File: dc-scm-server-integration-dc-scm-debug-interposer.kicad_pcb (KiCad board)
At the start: 6 copper layers, 90 x 62.3 mm, 166 parts, among them J1 Socket_DC-SCM-2.1_2x84_Rev-1-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, J10 PinHeader_2x5_P2.54mm_SMD, J11 PinHeader_2x5_P2.54mm_SMD, J12 PinHeader_2x5_P2.54mm_SMD, J13 PinHeader_2x5_P2.54mm_SMD, J15 Socket_SOP2-16_ACA-SPI-006-K0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, J16 Socket_SOP2-16_ACA-SPI-006-K0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, J17 PinHeader_2x5_P2.54mm_SMD, J2 PCB-Edge_DC-SCM-2.1_2x84_Rev-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, J3 PinHeader_2x5_P2.54mm_SMD, J4 PinHeader_2x5_P2.54mm_SMD, J5 PinHeader_2x5_P2.54mm_SMD, J6 PinHeader_2x5_P2.54mm_SMD, J7 PinHeader_2x5_P2.54mm_SMD, J9 PinHeader_2x5_P2.54mm_SMD, Q3 DMG1012T-7, U1 TLV76701_WSON

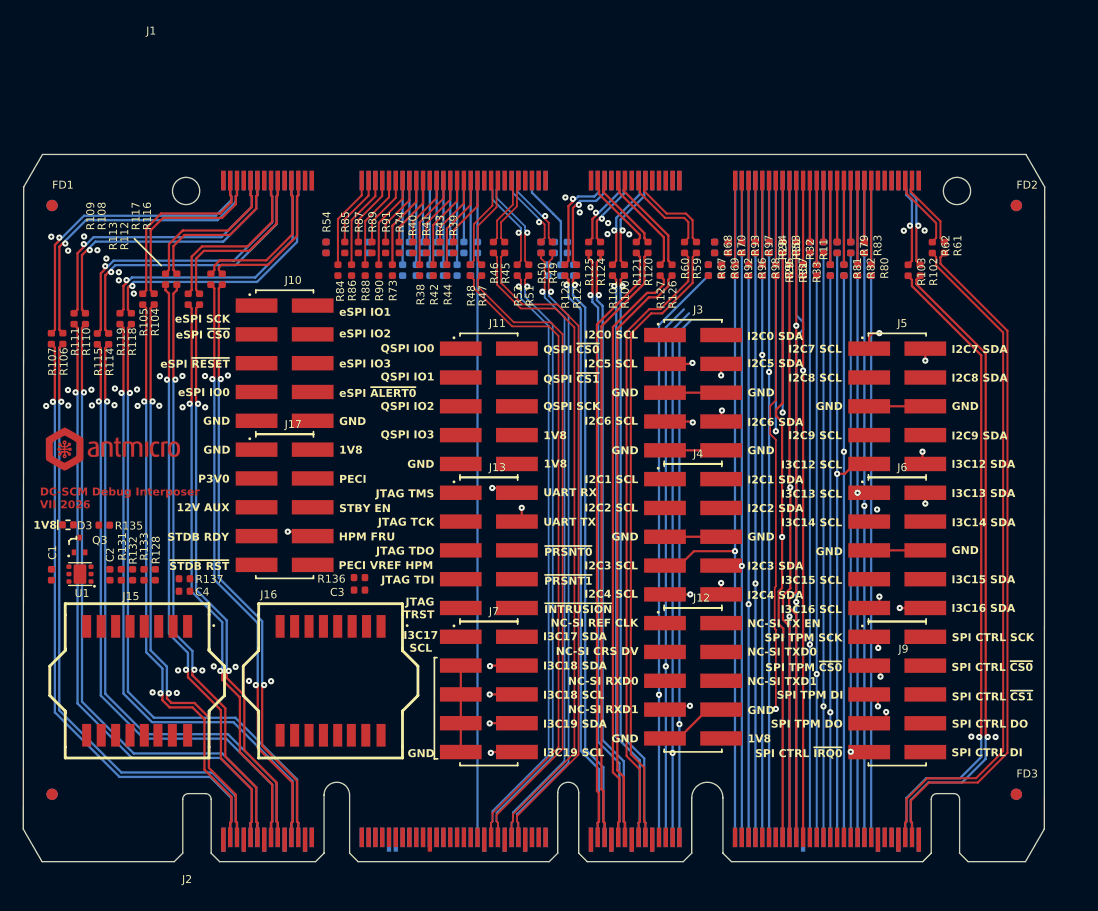
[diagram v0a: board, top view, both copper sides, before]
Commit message: [#100720] Continue routing low speeds
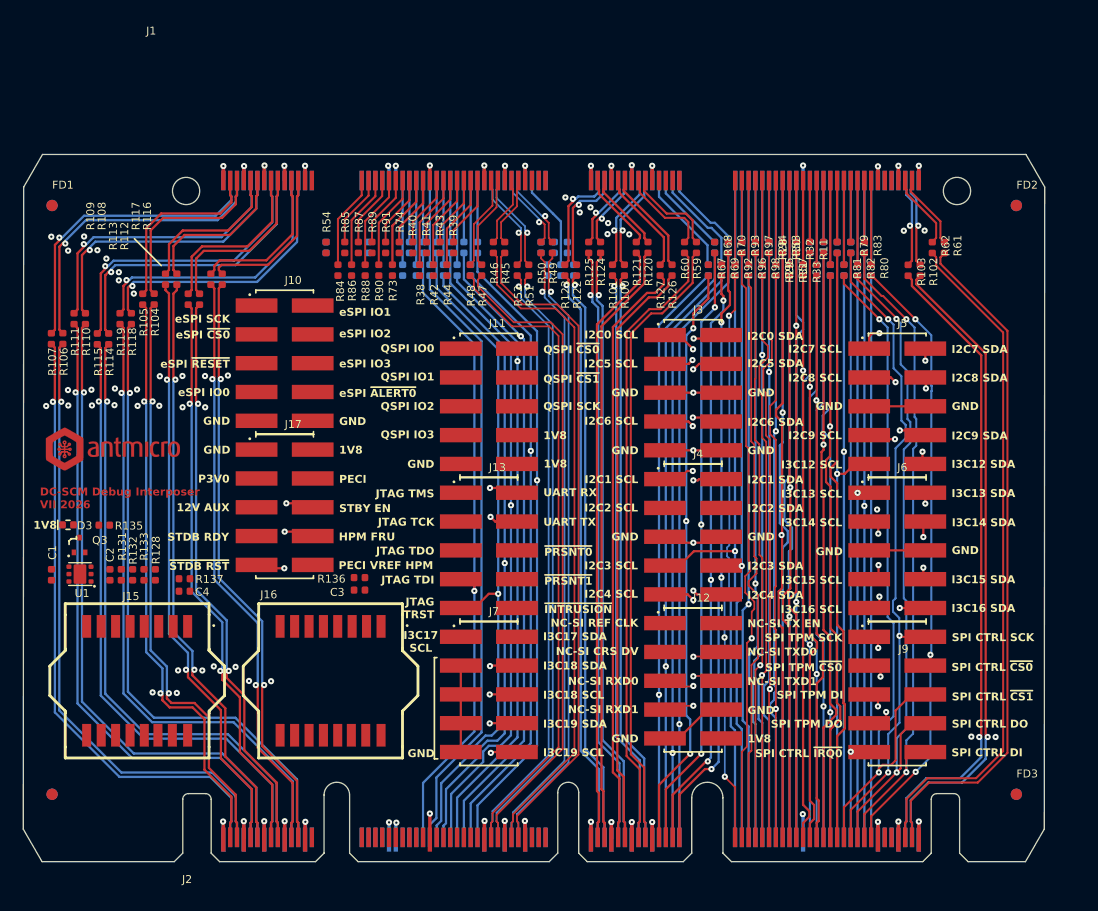
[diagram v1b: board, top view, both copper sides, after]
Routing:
- net GND: track 38.4 -> 138.9 mm, vias 42 -> 83
- net /DC-SCI edge connector/DC_SCM_STBY_EN: track 0.00 -> 78.9 mm, vias 0 -> 2
- net /DC-SCI edge connector/~{DC_SCM_STBY_RST}: track 0.00 -> 76.7 mm, vias 0 -> 2
- net /DC-SCI edge connector/DC_SCM_I2C_I3C14.SDA: track 0.00 -> 75.0 mm, vias 0 -> 4
- net /DC-SCI edge connector/DC_SCM_I2C0.SDA: track 0.00 -> 73.8 mm, vias 0 -> 2
- net /DC-SCI edge connector/DC_SCM_I2C_I3C15.SDA: track 0.00 -> 73.0 mm, vias 0 -> 4
- net /DC-SCI edge connector/DC_SCM_I2C0.SCL: track 0.00 -> 72.8 mm, vias 0 -> 2
- net /DC-SCI edge connector/DC_SCM_I2C1.SCL: track 0.00 -> 71.7 mm, vias 0 -> 2
- net /DC-SCI edge connector/DC_SCM_I2C_I3C14.SCL: track 0.00 -> 70.3 mm, vias 0 -> 4
- net /DC-SCI edge connector/DC_SCM_I2C_I3C15.SCL: track 0.00 -> 68.1 mm, vias 0 -> 4
- net /DC-SCI edge connector/DC_SCM_SPI_SCMCNTRL.~{CS1}: track 0.00 -> 62.9 mm, vias 0 -> 2
- net /DC-SCI edge connector/DC_SCM_I2C8.SCL: track 0.00 -> 62.6 mm, vias 0 -> 2
- net /DC-SCI edge connector/DC_SCM_NC-SI.RXD0: track 0.00 -> 61.8 mm, vias 0 -> 2
- net /DC-SCI edge connector/DC_SCM_I2C9.SCL: track 0.00 -> 61.5 mm, vias 0 -> 2
- net /DC-SCI edge connector/DC_SCM_I2C8.SDA: track 0.00 -> 61.2 mm, vias 0 -> 2
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- added copper zone on In1.Cu, net GND
- added copper zone on In2.Cu, net GND
- added copper zone on In4.Cu, net GND
